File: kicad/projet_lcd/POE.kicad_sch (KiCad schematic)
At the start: 79 parts, among them Q1 FOD817A3SD

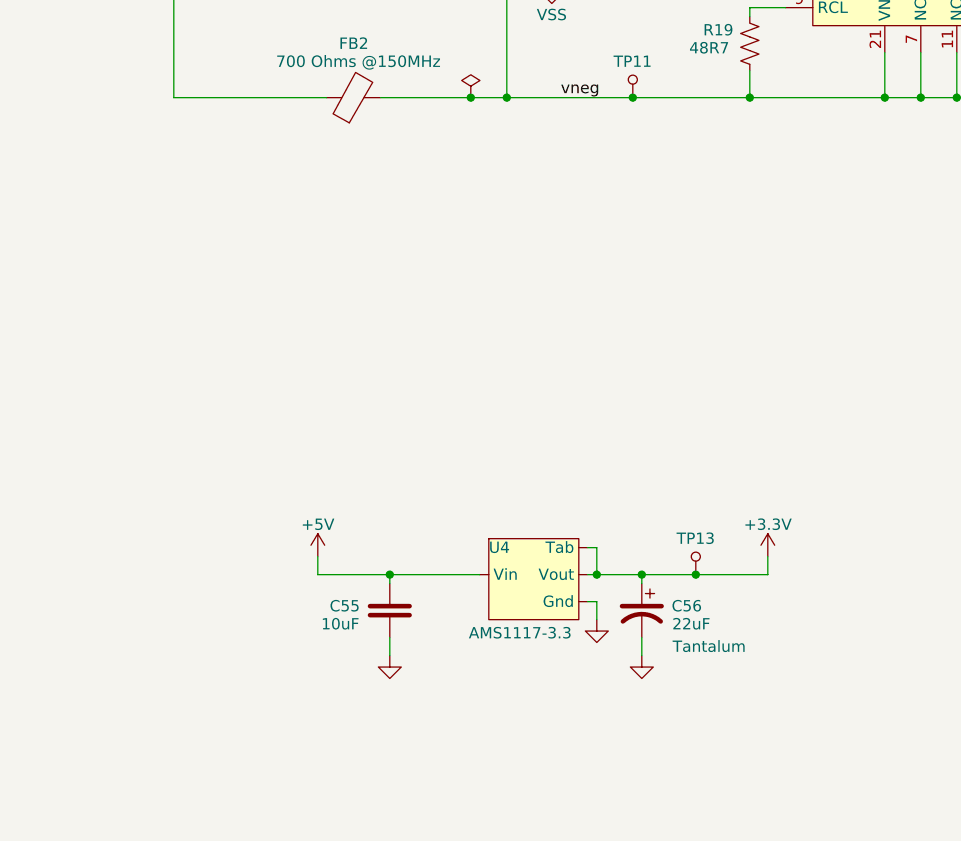
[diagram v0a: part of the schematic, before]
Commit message: cleanup
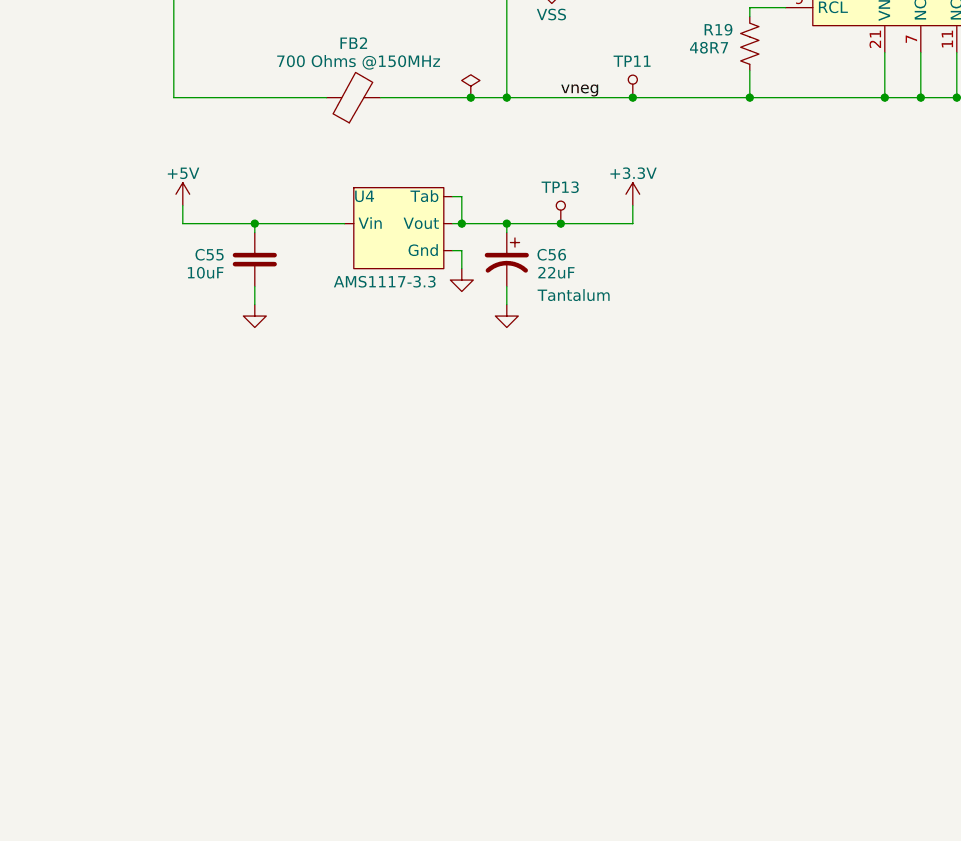
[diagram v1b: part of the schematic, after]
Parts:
- U3: footprint Voltage_Regulators:TL431 -> Voltage_regulators:TL431
- U4: footprint Voltage_Regulators:AMS1117-3.3 -> Voltage_regulators:AMS1117-3.3
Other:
- moved on the sheet: C55, C56, TP13, U4
